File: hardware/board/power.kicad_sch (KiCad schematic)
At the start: 23 parts, among them J1 POWER, SW1 POWER, U1 LD1117-3.3

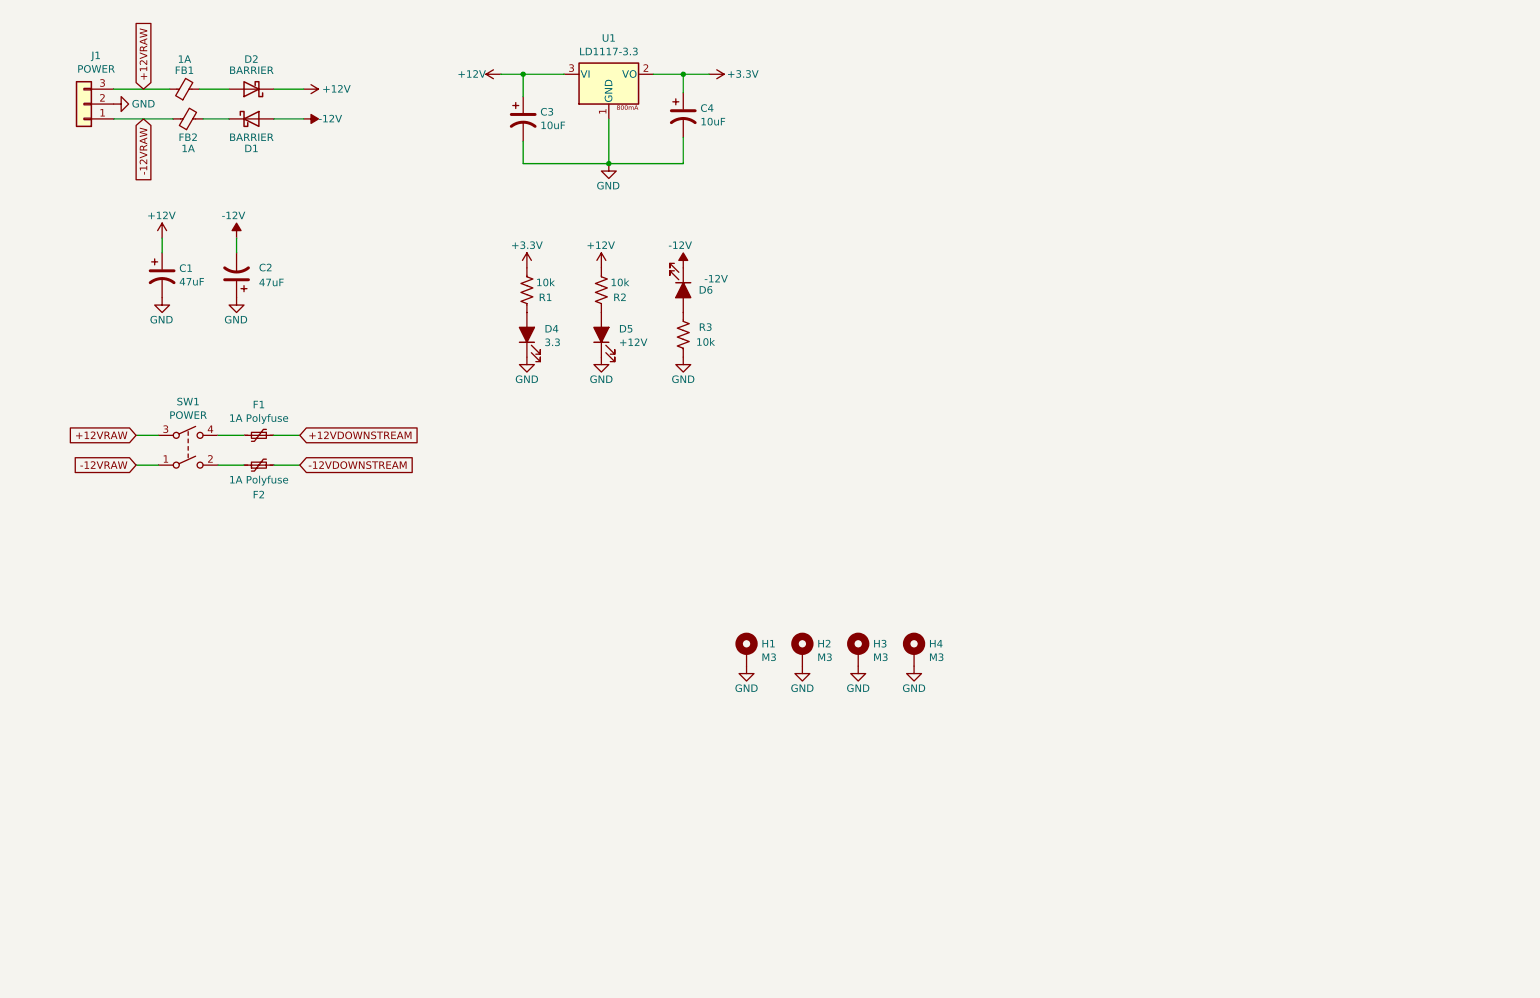
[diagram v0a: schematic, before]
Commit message: Initial stab at hardware revision
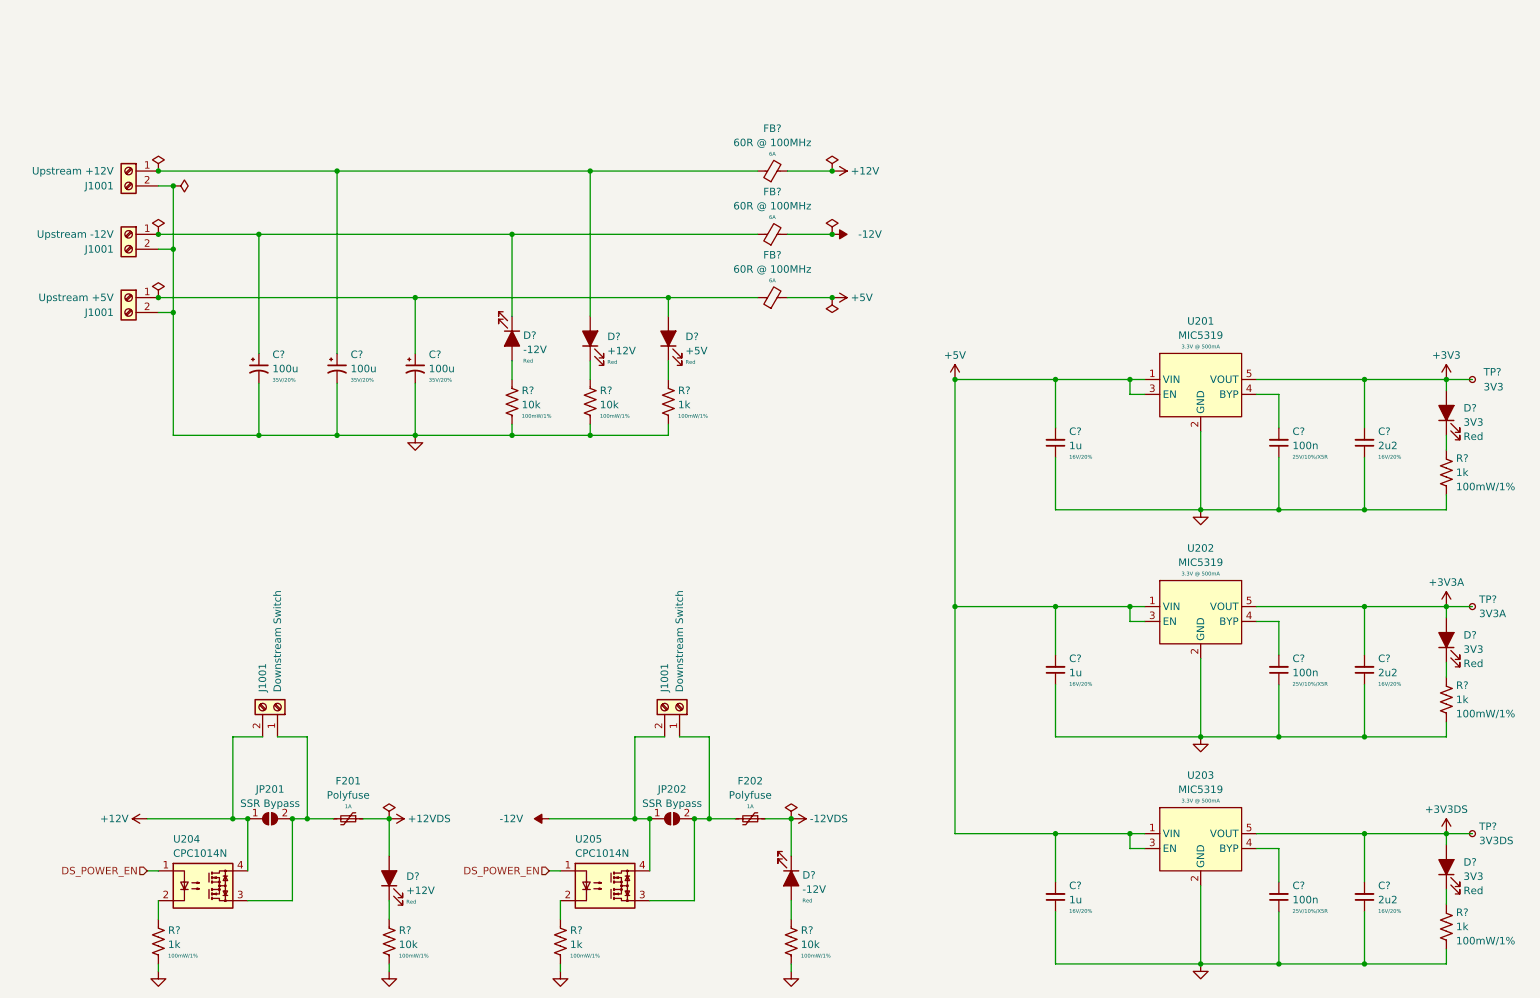
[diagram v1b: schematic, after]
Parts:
- removed C1, C2: 47uF, Capacitor_THT:CP_Radial_D5.0mm_P2.50mm, symbol Device:CP1
- removed C3, C4: 10uF, Capacitor_THT:CP_Radial_D5.0mm_P2.50mm, symbol Device:CP1
- removed D1, D2: BARRIER, winterbloom:DIODE_SOD-123_SOD-123F, symbol Diode:1N5819
- removed D4: 3.3, winterbloom:LED_0805_Kingbright_APT2012, symbol Device:LED_ALT
- removed D5: +12V, winterbloom:LED_0805_Kingbright_APT2012, symbol Device:LED_ALT
- removed D6: -12V, winterbloom:LED_0805_Kingbright_APT2012, symbol Device:LED_ALT
- removed F1, F2: 1A Polyfuse, winterbloom:Littelfuse_0805L, symbol Device:Polyfuse_Small
- removed FB1, FB2: 1A, Inductor_SMD:L_0603_1608Metric_Pad1.05x0.95mm_HandSolder, symbol Device:Ferrite_Bead_Small
- removed H1, H2, H3, H4: M3, MountingHole:MountingHole_3.2mm_M3_Pad_Via, symbol Mechanical:MountingHole_Pad
- removed J1: POWER, Connector_Wire:SolderWire-0.75sqmm_1x03_P4.8mm_D1.25mm_OD2.3mm, symbol Connector_Generic:Conn_01x03
- removed R1, R2, R3: 10k, Resistor_SMD:R_0603_1608Metric_Pad0.98x0.95mm_HandSolder, symbol Device:R_US
- removed SW1: POWER, Connector_Wire:SolderWire-0.75sqmm_1x04_P4.8mm_D1.25mm_OD2.3mm, symbol Switch:SW_DPST
- removed U1: LD1117-3.3, Package_TO_SOT_SMD:SOT-223-3_TabPin2, symbol winterbloom:LM1117-3.3
- added C? (x3): 100u, Capacitor_SMD:CP_Elec_6.3x9.9, symbol Device:C_Polarized_Small_US
- added C? (x3): 1u, winterbloom:C_0603_HandSolder, symbol Device:C_Small
- added C? (x3): 100n, winterbloom:C_0603_HandSolder, symbol Device:C_Small
- added C? (x3): 2u2, winterbloom:C_0603_HandSolder, symbol Device:C_Small
- added D? (x3): 3V3, winterbloom:LED_0805_Kingbright_APT2012, symbol Device:LED_Filled
- added D? (x2): -12V, winterbloom:LED_0805_Kingbright_APT2012, symbol Device:LED_Filled
- added D? (x2): +12V, winterbloom:LED_0805_Kingbright_APT2012, symbol Device:LED_Filled
- added D?: +5V, winterbloom:LED_0805_Kingbright_APT2012, symbol Device:LED_Filled
- added F201, F202: Polyfuse, winterbloom:Fuse_Littelfuse_0805L, symbol Device:Polyfuse_Small
- added FB? (x3): 60R @ 100MHz, Inductor_SMD:L_1806_4516Metric_Pad1.45x1.90mm_HandSolder, symbol Device:FerriteBead_Small
- added J1001: Upstream +12V, winterbloom:TerminalBlock_4UCON_1x02_P3.50mm_Horizontal, symbol Connector:Screw_Terminal_01x02
- added J1001 (x2): Downstream Switch, winterbloom:TerminalBlock_4UCON_1x02_P3.50mm_Horizontal, symbol Connector:Screw_Terminal_01x02
- added J1001: Upstream -12V, winterbloom:TerminalBlock_4UCON_1x02_P3.50mm_Horizontal, symbol Connector:Screw_Terminal_01x02
- added J1001: Upstream +5V, winterbloom:TerminalBlock_4UCON_1x02_P3.50mm_Horizontal, symbol Connector:Screw_Terminal_01x02
- added JP201, JP202: SSR Bypass, Jumper:SolderJumper-2_P1.3mm_Open_Pad1.0x1.5mm, symbol Jumper:SolderJumper_2_Open
- added R? (x4): 10k, winterbloom:R_0603_HandSolder, symbol Device:R_US
- added R? (x6): 1k, winterbloom:R_0603_HandSolder, symbol Device:R_US
- added TP?: 3V3DS, TestPoint:TestPoint_Pad_D1.0mm, symbol Connector:TestPoint_Small
- added TP?: 3V3A, TestPoint:TestPoint_Pad_D1.0mm, symbol Connector:TestPoint_Small
- added TP?: 3V3, TestPoint:TestPoint_Pad_D1.0mm, symbol Connector:TestPoint_Small
- added U201, U202, U203: MIC5319, Package_TO_SOT_SMD:SOT-23-5, symbol winterbloom:MIC5319
- added U204, U205: CPC1014N, Package_SO:SOP-4_3.8x4.1mm_P2.54mm, symbol Relay_SolidState:CPC1017N
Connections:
- net +12V: now also FB?.2, J1001.2 (Pin_2), JP201.1 (A), U204.4
- net +3V3: now also C?.2, D?.2 (A), TP?.1, U201.5 (VOUT)
- net -12V: now also FB?.2, J1001.2 (Pin_2), JP202.1 (A), U205.4
- net GND: now also C?.1, C?.1, C?.1, C?.1, C?.1, C?.1, C?.1, C?.1, C?.1, C?.2, C?.2, C?.2, J1001.2 (Pin_2), J1001.2 (Pin_2), J1001.2 (Pin_2), R?.2, R?.2, R?.2, R?.2, R?.2, R?.2, R?.2, R?.2, R?.2, R?.2, U201.2 (GND), U202.2 (GND), U203.2 (GND)
- new net: C?.1, D?.2 (A), FB?.1, J1001.1 (Pin_1) (x2)
- new net: D?.2 (A), R?.1 (x2)
- new net: R?.1, U204.2
- new net: C?.2, U203.4 (BYP)
- new net: C?.1, D?.1 (K), FB?.1, J1001.1 (Pin_1)
- new net: F201.2, J1001.1 (Pin_1), JP201.2 (B), U204.3
- new net: C?.2, U202.4 (BYP)
- new net: D?.1 (K), R?.1 (x6)
- new net: C?.2, U201.4 (BYP)
- new net: R?.1, U205.2
- new net: F202.2, J1001.1 (Pin_1), JP202.2 (B), U205.3
- new net +12VDS: D?.2 (A), F201.1
- new net +3V3A: C?.2, D?.2 (A), TP?.1, U202.5 (VOUT)
- new net +3V3DS: C?.2, D?.2 (A), TP?.1, U203.5 (VOUT)
- new net +5V: C?.2, C?.2, C?.2, FB?.2, U201.1 (VIN), U201.3 (EN), U202.1 (VIN), U202.3 (EN), U203.1 (VIN), U203.3 (EN)
- new net -12VDS: D?.1 (K), F202.1
- new net DS_POWER_EN: U204.1, U205.1
